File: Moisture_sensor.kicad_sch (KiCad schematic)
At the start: 3 parts, among them J1 Conn_01x02_Socket, U2 TLV2371DBV

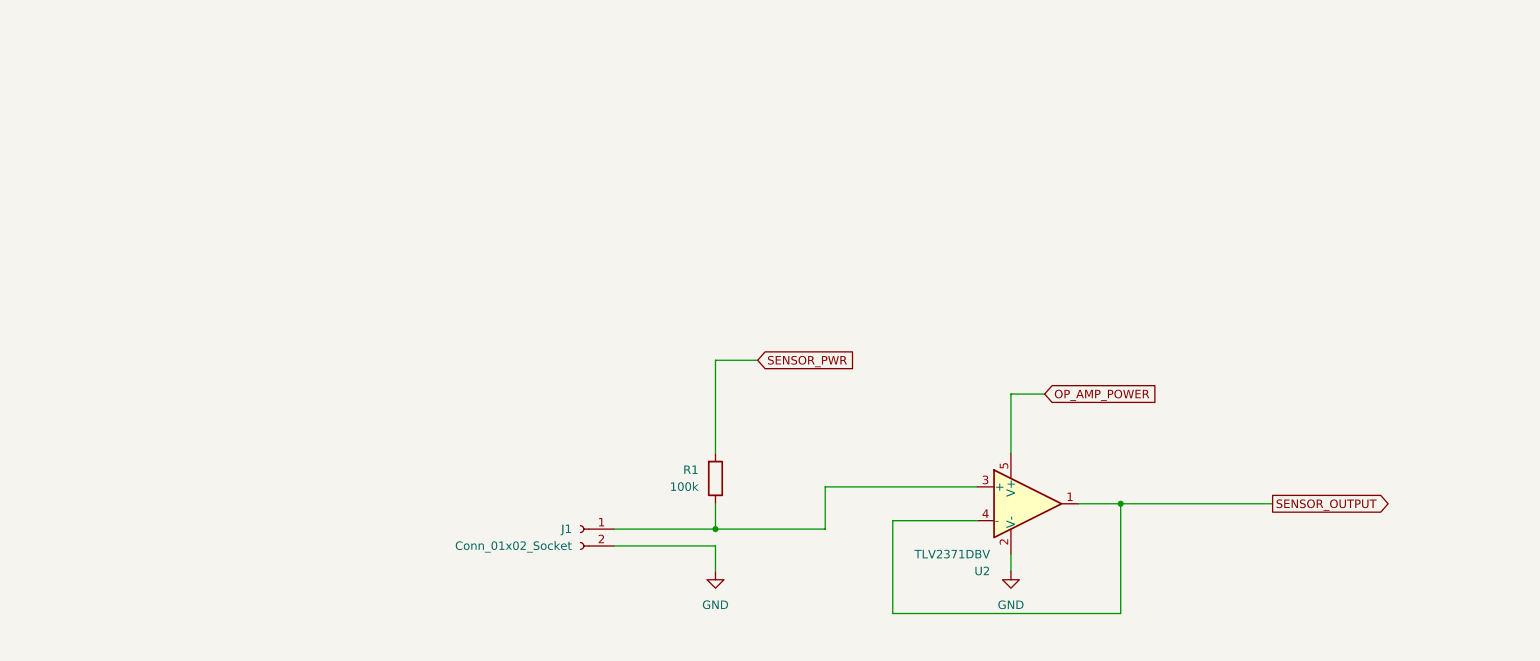
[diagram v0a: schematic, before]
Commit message: Completed first iteration and reviews
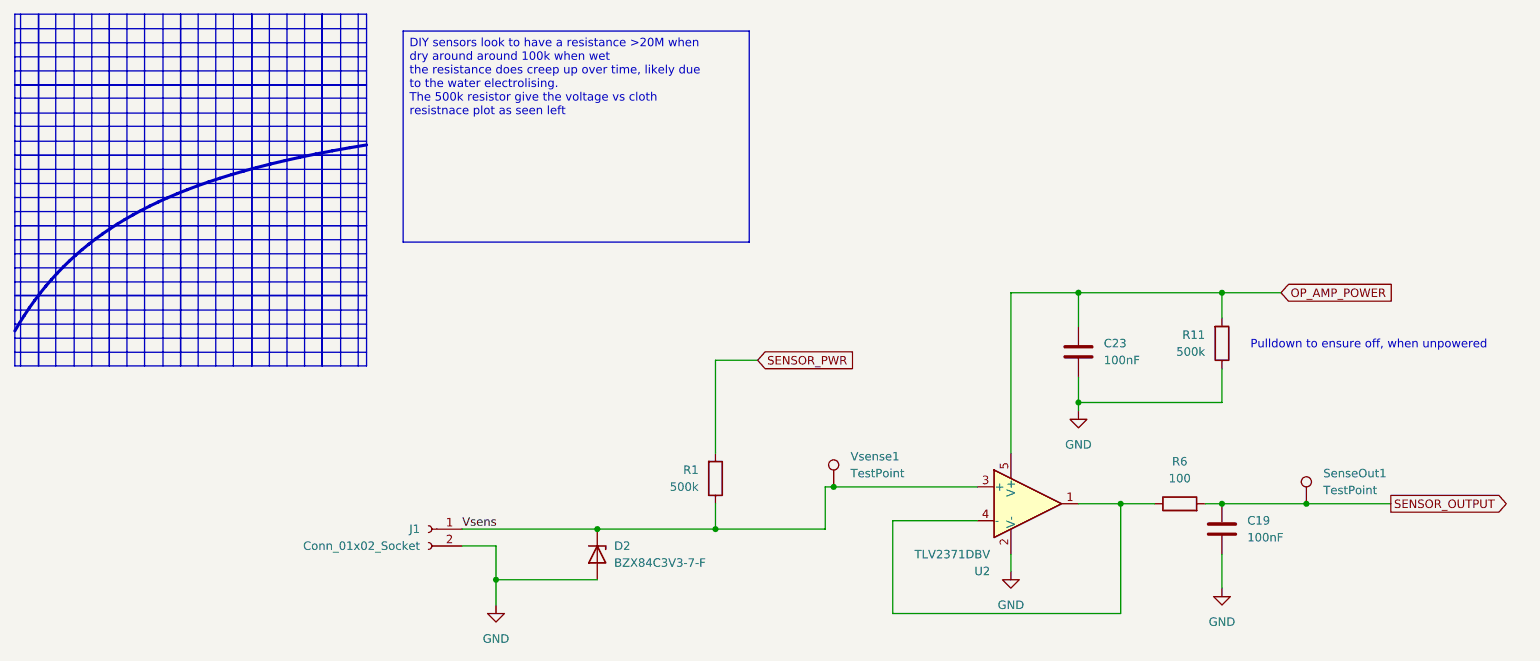
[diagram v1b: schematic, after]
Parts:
- added C19, C23: 100nF, Capacitor_SMD:C_0805_2012Metric_Pad1.18x1.45mm_HandSolder, symbol Device:C
- added D2: BZX84C3V3-7-F, Package_TO_SOT_SMD:SOT-23, symbol Diode:BZX84Cxx
- added R11: 500k, Resistor_SMD:R_0805_2012Metric_Pad1.20x1.40mm_HandSolder, symbol Device:R
- added R6: 100, Resistor_SMD:R_0805_2012Metric_Pad1.20x1.40mm_HandSolder, symbol Device:R
- added SenseOut1, Vsense1: TestPoint, TestPoint:TestPoint_Pad_D1.0mm, symbol Connector:TestPoint
- J1: footprint (none) -> Connector_Wire:SolderWire-0.1sqmm_1x02_P3.6mm_D0.4mm_OD1mm_Relief
- R1: value 100k -> 500k; footprint (none) -> Resistor_SMD:R_0805_2012Metric_Pad1.20x1.40mm_HandSolder; Supplier (none) -> Digikey; Supplier Part Number (none) -> 738-RNCF0805BTE500KCT-ND
- U2: Supplier (none) -> Digikey; Supplier Part Number (none) -> 296-13057-1-ND
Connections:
- net GND: now also C19.2, C23.2, D2.1 (A), R11.1
- net OP_AMP_POWER: now also C23.1, R11.2
- net SENSOR_OUTPUT: now also C19.1, R6.2, SenseOut1.1; no longer U2.1, U2.4 (-)
- net Vsens: now reaches J1.1 (Pin_1), R1.1, U2.3 (+)
- net Vsens: now also D2.3 (K), Vsense1.1
- new net: R6.1, U2.1, U2.4 (-)
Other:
- note added: "Pulldown to ensure off, when unpowered"
- company: (none) -> Horatio Pistachio
- title: (none) -> WashingLineMonitor-P0001
- moved on the sheet: J1

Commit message: commit of local files before designing next version
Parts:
- D2: JLC_Part_Number (none) -> C177019
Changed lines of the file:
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@@
+			)
+		)
+		(property "JLC_Part_Number" ""
+			(at 193.04 88.9 90)
+			(effects
+				(font
+					(size 1.27 1.27)
+				)
+				(hide yes)
 			)
 		)
@@
 		)
 		(property "Supplier Part Number" "BZX84C3V3-FDICT-ND"
+			(at 105.41 96.52 90)
+			(effects
+				(font
+					(size 1.27 1.27)
+				)
+				(hide yes)
+			)
+		)
+		(property "JLC_Part_Number" "C177019"
 			(at 105.41 96.52 90)
 			(effects
@@
 			)
 		)
+		(property "JLC_Part_Number" ""
+			(at 123.19 85.09 0)
+			(effects
+				(font
+					(size 1.27 1.27)
+				)
+				(hide yes)
+			)
+		)
 		(pin "1"
 		)
@@
 			)
 		)
+		(property "JLC_Part_Number" ""
+			(at 199.39 64.77 0)
+			(effects
+				(font
+					(size 1.27 1.27)
+				)
+				(hide yes)
+			)
+		)
 		(pin "1"
 		)
@@
 		)
 		(property "Supplier" "Digikey"
+			(at 170.18 88.9 0)
+			(effects
+				(font
+					(size 1.27 1.27)
+				)
+				(hide yes)
+			)
+		)
+		(property "JLC_Part_Number" ""
 			(at 170.18 88.9 0)
 			(effects
@@
 			)
 		)
+		(property "JLC_Part_Number" ""
+			(at 212.09 88.9 0)
+			(effects
+				(font
+					(size 1.27 1.27)
+				)
+				(hide yes)
+			)
+		)
 		(pin "1"
 		)
@@
 			)
 		)
+		(property "JLC_Part_Number" ""
+			(at 177.8 66.04 0)
+			(effects
+				(font
+					(size 1.27 1.27)
+				)
+				(hide yes)
+			)
+		)
 		(pin "1"
 		)
@@
 			)
 		)
+		(property "JLC_Part_Number" ""
+			(at 199.39 92.71 0)
+			(effects
+				(font
+					(size 1.27 1.27)
+				)
+				(hide yes)
+			)
+		)
 		(pin "1"
 		)
@@
 		)
 		(property "Description" "test point"
+			(at 140.97 86.36 0)
+			(effects
+				(font
+					(size 1.27 1.27)
+				)
+				(hide yes)
+			)
+		)
+		(property "JLC_Part_Number" ""
 			(at 140.97 86.36 0)
 			(effects
@@
 			(at 80.01 92.71 0)
 			(effects
+				(font
+					(size 1.27 1.27)
+				)
+				(hide yes)
+			)
+		)
+		(property "JLC_Part_Number" ""
+			(at 80.01 92.71 0)
+			(effects
